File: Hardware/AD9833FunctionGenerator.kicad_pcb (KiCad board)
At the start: 2 copper layers, 110.6 x 174.6 mm, 54 parts, among them U1 LM7805_TO220

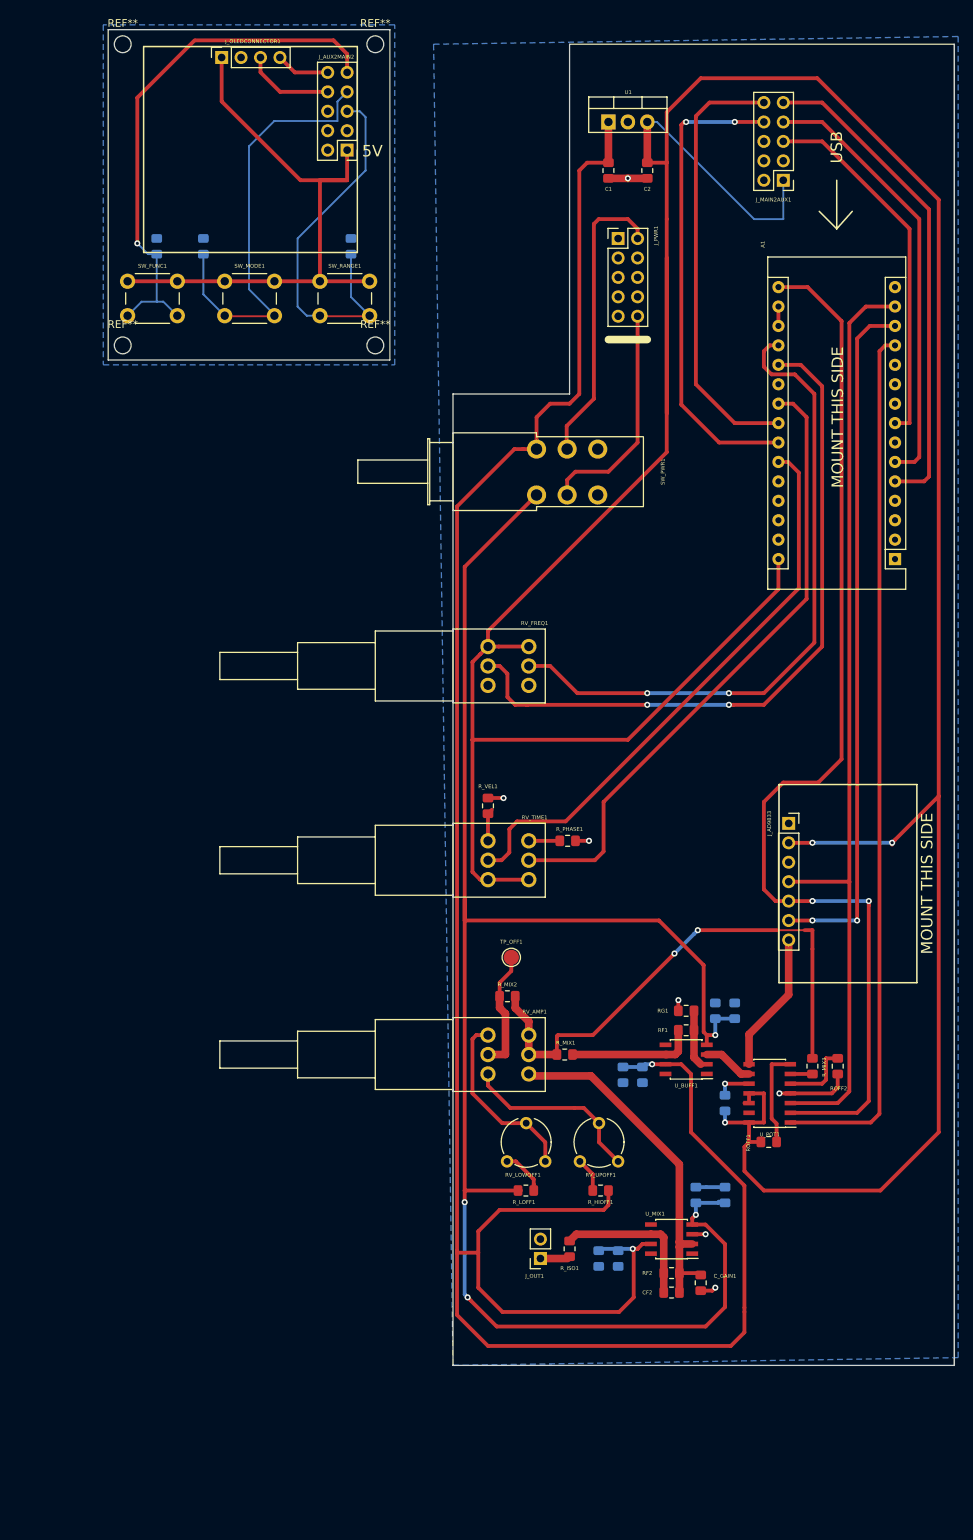
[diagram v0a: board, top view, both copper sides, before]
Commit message: Draft RevA Board
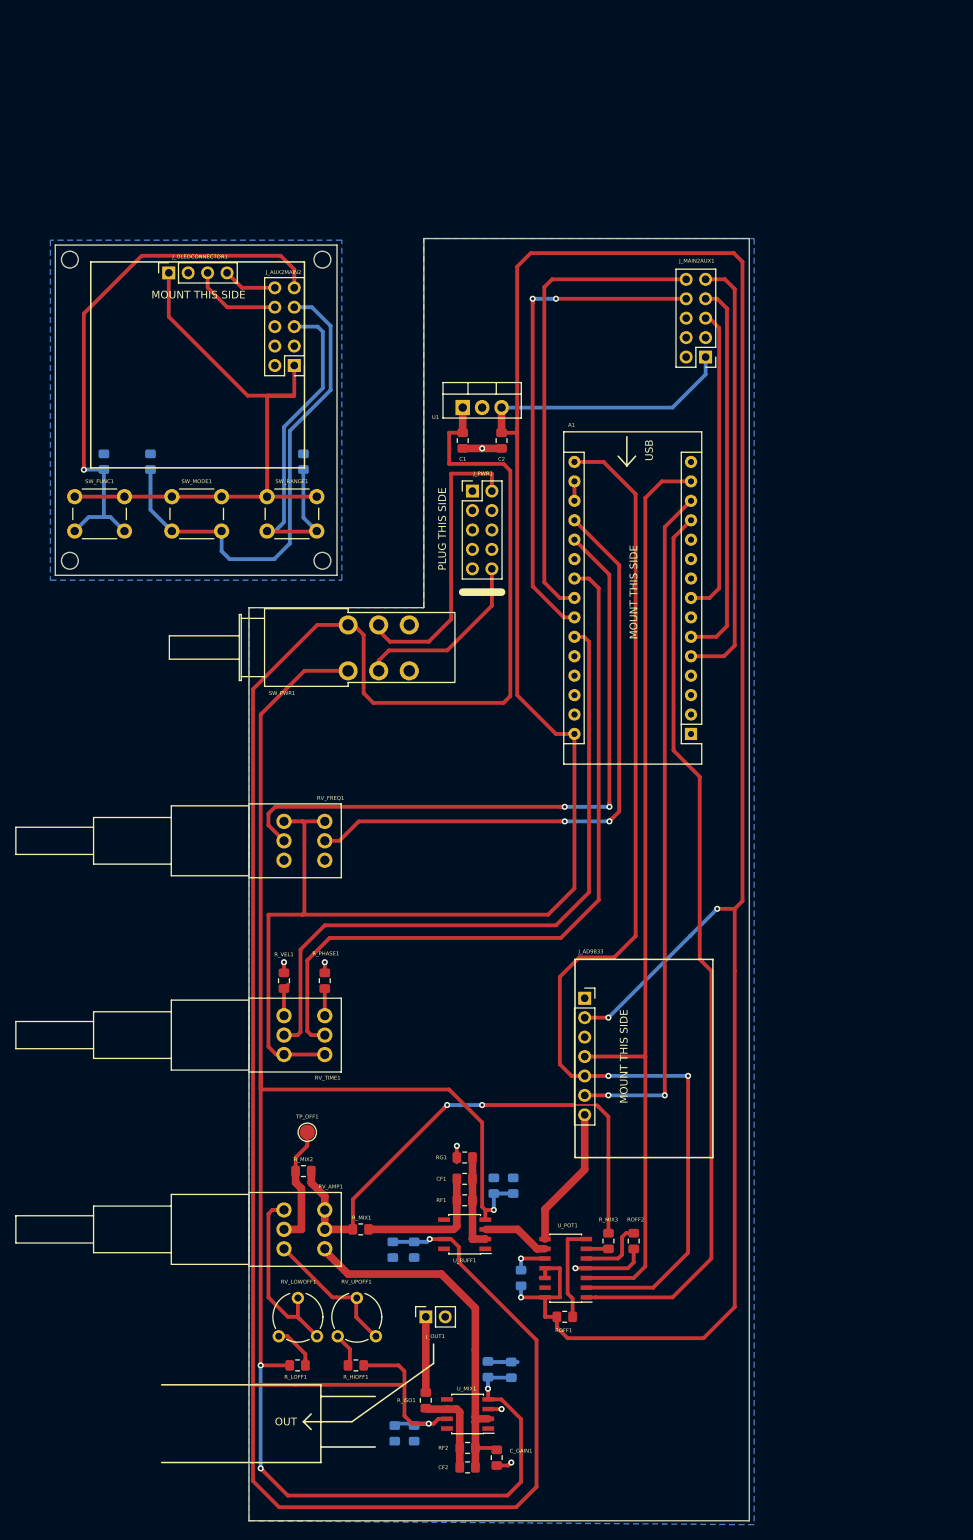
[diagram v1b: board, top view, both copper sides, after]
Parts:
- added CF1: 2pF, Capacitor_SMD:C_0805_2012Metric_Pad1.15x1.40mm_HandSolder, F.Cu at (95.5, 186.4)
- moved U1 41.9 mm to (95.2, 85.6)
- moved C1 40.1 mm to (95.2, 89.9)
- moved C2 40.1 mm to (100.3, 89.9)
- moved R_HIOFF1 39.3 mm to (81.3, 210.8)
- moved RV_UPOFF1 39.1 mm to (83.9, 207.0)
- moved J_PWR1 38.1 mm to (96.5, 96.5)
- moved C_BUFFBP1 37.8 mm to (86.1, 195.7)
- moved C_BUFFBP2 37.6 mm to (88.9, 195.7)
- moved RV_LOWOFF1 37.6 mm to (76.2, 207.0)
- moved R_LOFF1 37.6 mm to (73.7, 210.8)
- moved C_BUFFBP3 36.9 mm to (99.3, 187.3)
- moved U_BUFF1 36.9 mm to (95.5, 193.7)
- moved C_BUFFBP4 36.9 mm to (101.9, 187.3)
- moved R_PHASE1 36.6 mm to (77.2, 160.5), turned to 270 degrees
- moved RF1 36.5 mm to (95.5, 189.2)
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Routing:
- net /5V: track 472.0 -> 446.0 mm
- net /PHASE1: track 82.4 -> 97.6 mm
- net /VEL1: track 75.5 -> 88.9 mm
- net /AuxiliaryBoard/MODEBTN_AUX: track 56.2 -> 64.6 mm
- net Net-(CF2-Pad1): track 20.1 -> 11.9 mm
- net /RANGEBTN: track 48.5 -> 40.5 mm
- net /MODEBTN: track 57.6 -> 50.1 mm
- net /WAVEBTN: track 64.5 -> 57.2 mm
- net /OutputSection/SIGOUT: track 3.91 -> 10.0 mm
- net Net-(RV_AMP1-Pad1): track 24.1 -> 18.1 mm
- net /FREQHI: track 86.4 -> 80.6 mm
- net Net-(J_PWR1-Pad10): track 29.7 -> 23.9 mm
- net /FREQLO: track 91.7 -> 86.2 mm
- net /SDA: track 57.6 -> 62.3 mm
- net /SCK: track 142.7 -> 146.8 mm
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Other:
- board size 110.6 x 174.6 mm -> 90.7 x 167.6 mm
- board text added: "OUT"
- board text added: "PLUG THIS SIDE"
- board text removed: "5V"
